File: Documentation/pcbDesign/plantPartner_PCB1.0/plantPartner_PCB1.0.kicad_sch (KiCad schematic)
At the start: 52 parts, among them IC1 MPM3610, J1 Conn_01x04, J10 Screw_Terminal, J2 Conn_01x04, J3 Conn_01x04, J4 Screw_Terminal, J5 Screw_Terminal, J6 Screw_Terminal, J7 Conn_01x03, J8 Screw_Terminal, J9 Conn_01x03, K1 SRD-05VDC-SL-C, K2 SRD-05VDC-SL-C, Q1 PNP, Q2 PNP, U1 ESP32-WROOM-32, U2 MAX485

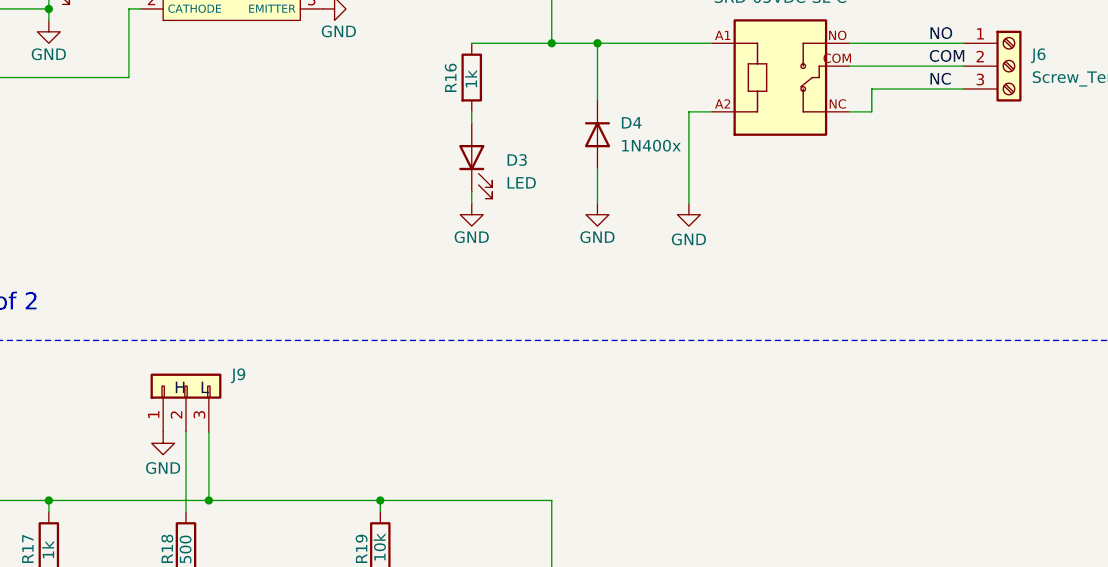
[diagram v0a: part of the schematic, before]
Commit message: Added hours from meeting today and winter break
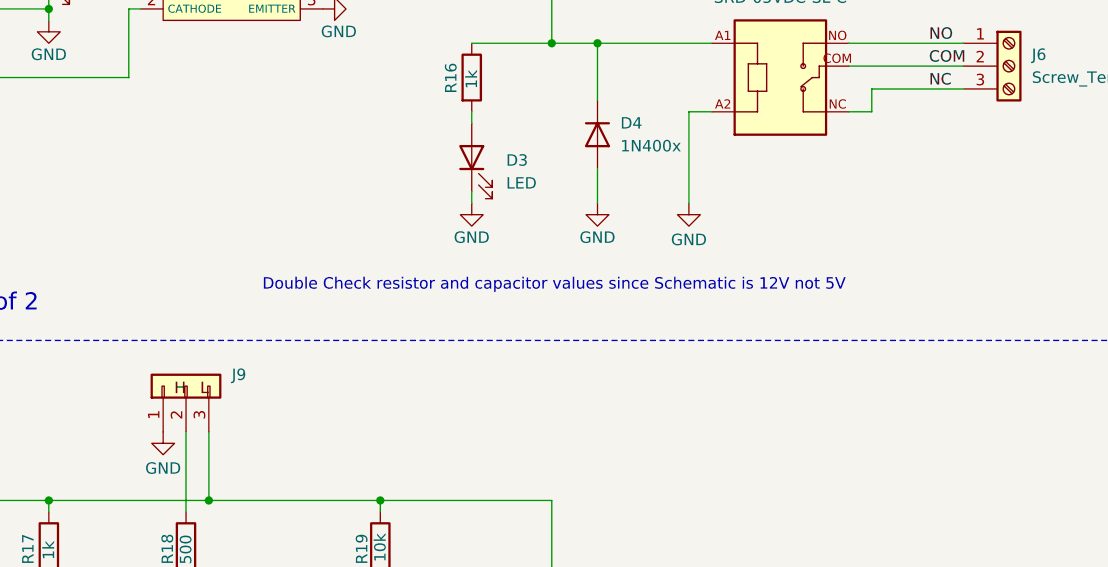
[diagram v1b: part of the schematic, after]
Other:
- note added: "Double Check resistor and capacitor values since Schematic is 12V not 5V"
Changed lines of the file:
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@@
+		)
+	)
+	(text "Double Check resistor and capacitor values since Schematic is 12V not 5V\n"
+		(exclude_from_sim no)
+		(at 197.104 81.534 0)
+		(effects
+			(font
+				(size 1.27 1.27)
+			)
 		)
 	)
